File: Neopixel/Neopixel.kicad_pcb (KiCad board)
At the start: 2 copper layers, 2 parts, among them J1 Screw_Terminal_01x03

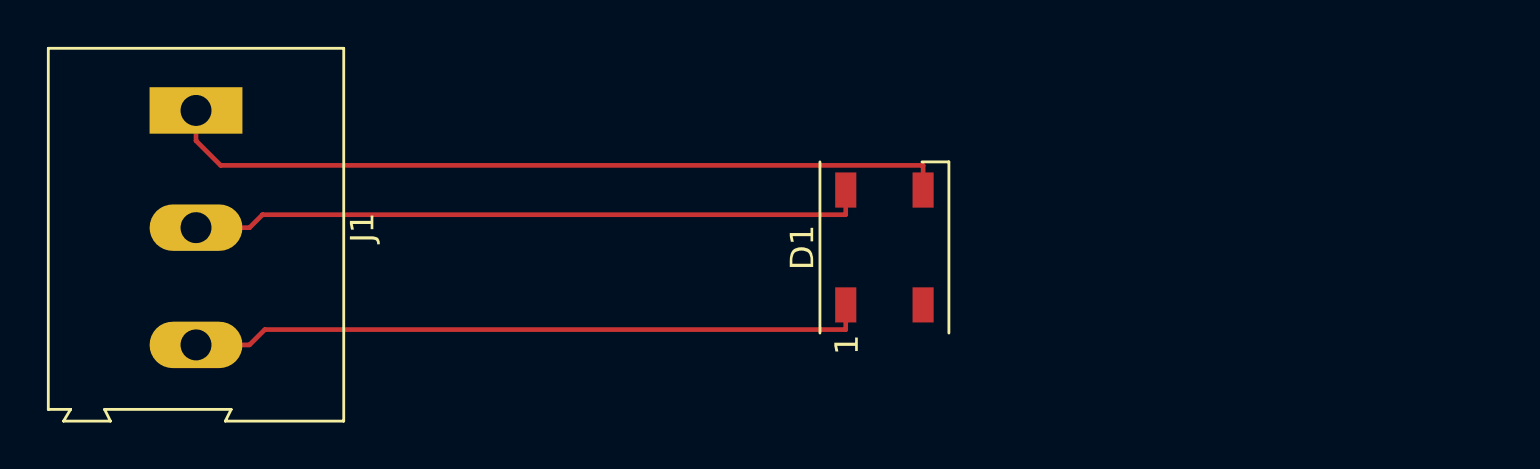
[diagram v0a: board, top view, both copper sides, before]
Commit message: designing
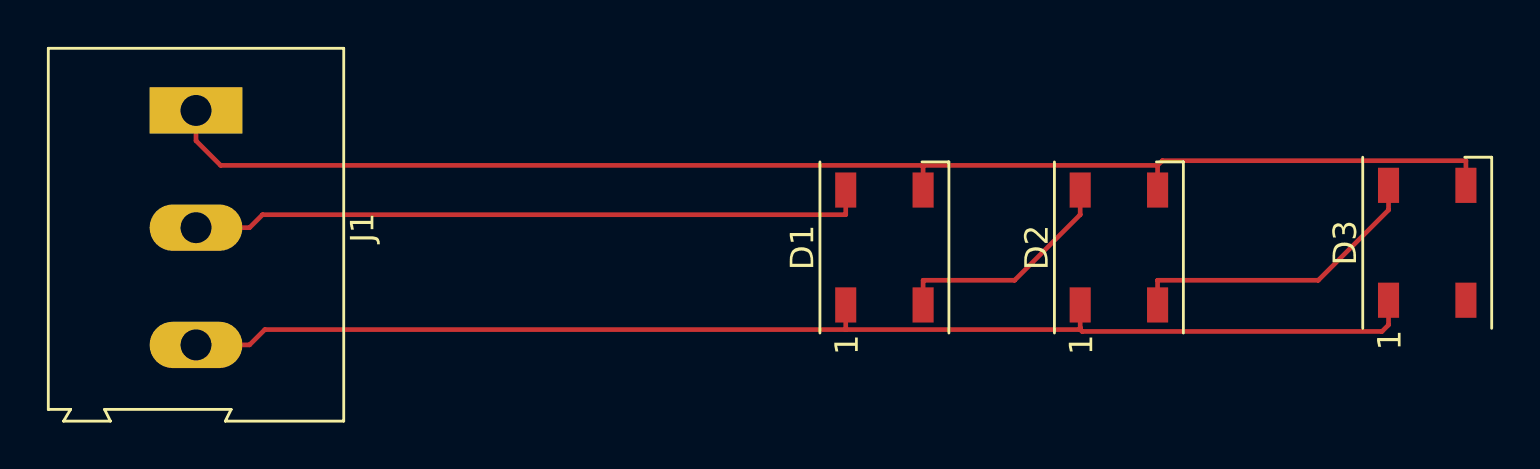
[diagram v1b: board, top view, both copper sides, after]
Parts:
- added D2: WS2812B, LED_SMD:LED_WS2812B_PLCC4_5.0x5.0mm_P3.2mm, F.Cu at (97.8, 71.0)
- added D3: WS2812B, LED_SMD:LED_WS2812B_PLCC4_5.0x5.0mm_P3.2mm, F.Cu at (111.0, 70.8)
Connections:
- D1 pad 2: unconnected-(D1-DOUT-Pad2) -> Net-(D1-DOUT)
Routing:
- net +5V: track 29.0 -> 54.4 mm
- net GND: track 33.8 -> 59.1 mm
- net Net-(D2-DOUT): track 0.00 -> 13.2 mm
- net Net-(D1-DOUT): track 0.00 -> 9.96 mm
